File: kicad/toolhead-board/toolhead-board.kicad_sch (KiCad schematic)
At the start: 46 parts, among them J1 Conn_02x12_Top_Bottom, J10 CAM, J11 DB9_Male_MountingHoles, J12 Conn_01x08, J2 ZM, J3 LM, J4 RM, J5 RGB, J6 VL, J7 VR, J8 ZES, J9 USB_C_Receptacle_USB2.0, U1 XGZP6857A100KPGPN, U2 XGZP6857A100KPGPN, U3 MIC5233-5.0YM5-TR, U4 74LVC1G17GW, U5 LMZM23601

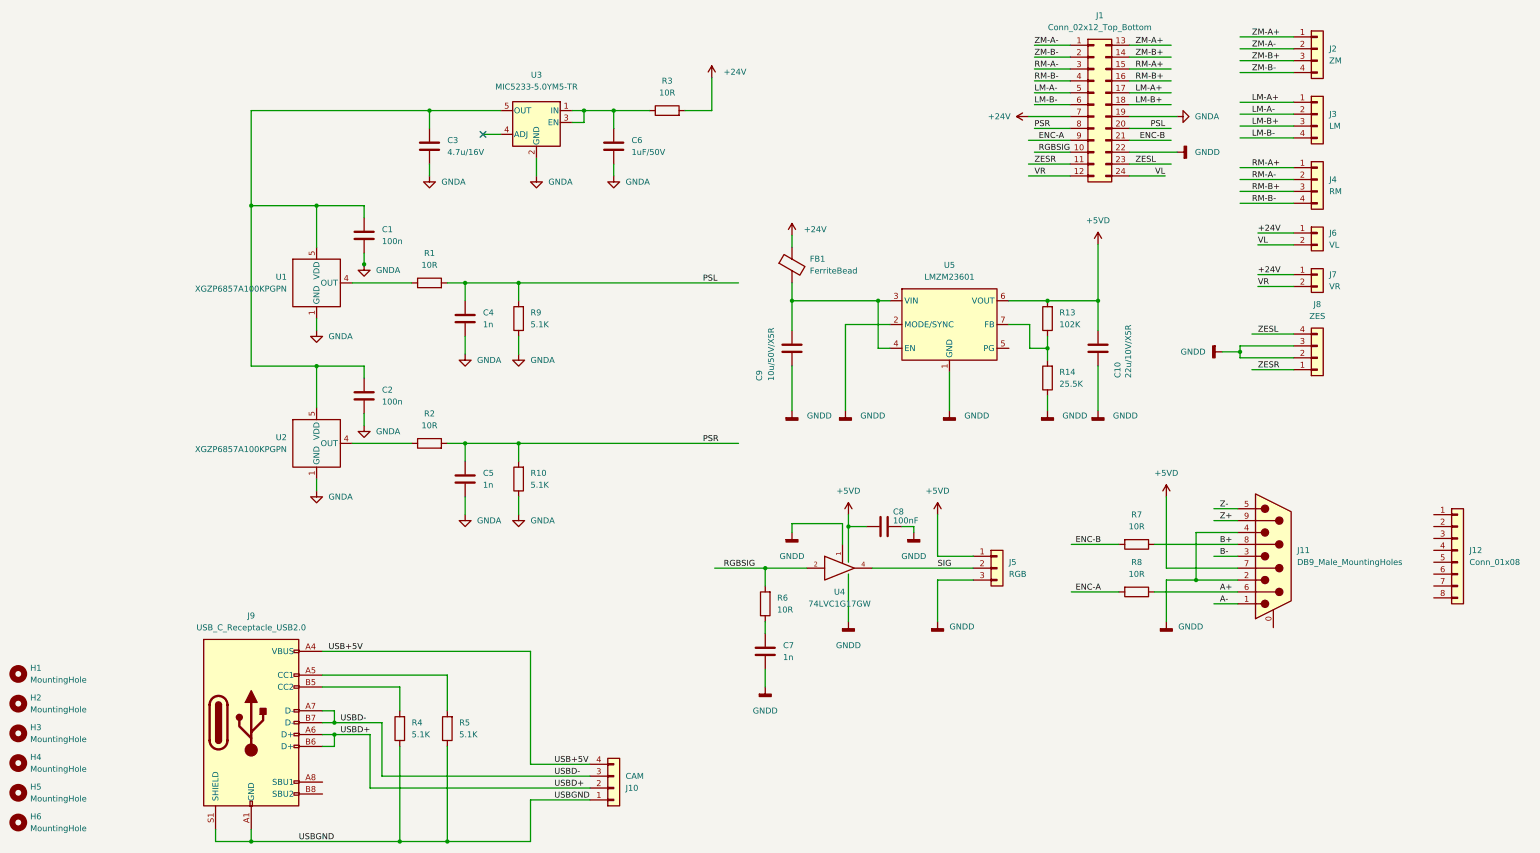
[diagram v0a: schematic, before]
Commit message: Added RS422 receiver
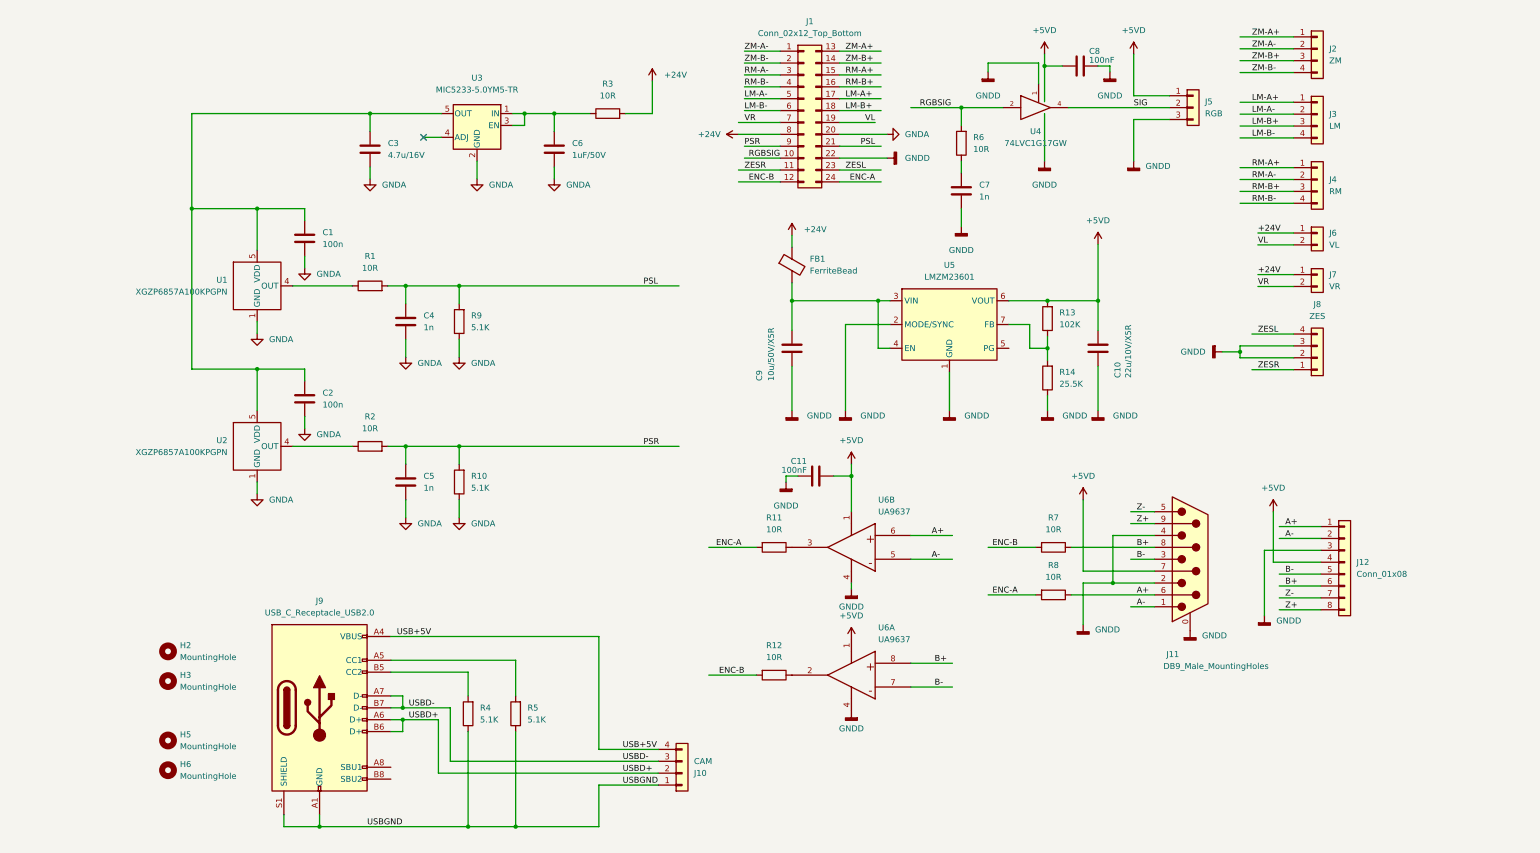
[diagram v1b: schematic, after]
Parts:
- removed H1, H4: MountingHole, Project:MountingHole_3.2mm_M3, symbol Mechanical:MountingHole
- added C11: 100nF, Capacitor_SMD:C_0603_1608Metric, symbol Device:C
- added R11, R12: 10R, Resistor_SMD:R_0805_2012Metric, symbol Device:R
- added U6: UA9637, Package_SO:SO-8_3.9x4.9mm_P1.27mm, symbol Interface_LineDriver:UA9637
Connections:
- net +24V: now also J1.8 (Pin_8); no longer J1.7 (Pin_7)
- net +5VD: now also J12.4 (Pin_4), C11.1, U6.1 (VCC), U6.1 (VCC)
- net A+: now also J12.1 (Pin_1), U6.6 (IN+)
- net A-: now also J12.2 (Pin_2), U6.5 (IN-)
- net B+: now also J12.6 (Pin_6), U6.8 (IN+)
- net B-: now also J12.5 (Pin_5), U6.7 (IN-)
- net ENC-A: now also J1.24 (Pin_24), R11.2; no longer J1.9 (Pin_9)
- net ENC-B: now also J1.12 (Pin_12), R12.2; no longer J1.21 (Pin_21)
- net GND: now also J11.0 (PAD), J12.3 (Pin_3), C11.2, U6.4 (GND), U6.4 (GND)
- net GNDA: now also J1.20 (Pin_20); no longer J1.19 (Pin_19)
- net PSL: now also J1.21 (Pin_21); no longer J1.20 (Pin_20)
- net PSR: now also J1.9 (Pin_9); no longer J1.8 (Pin_8)
- net VL: now also J1.19 (Pin_19); no longer J1.24 (Pin_24)
- net VR: now also J1.7 (Pin_7); no longer J1.12 (Pin_12)
- net Z+: now also J12.8 (Pin_8)
- net Z-: now also J12.7 (Pin_7)
- new net: R12.1, U6.2 (OUT)
- new net: R11.1, U6.3 (OUT)
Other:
- moved on the sheet: C1, C2, C3, C4, C5, C6, C7, C8, H2, H3, H5, H6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
